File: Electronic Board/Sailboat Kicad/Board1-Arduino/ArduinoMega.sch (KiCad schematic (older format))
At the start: 7 parts, among them J2 Conn_01x08, J3 Conn_01x08, J4 Conn_01x08, J5 Conn_02x18_Odd_Even, J6 Conn_01x08, J7 Conn_01x08, J8 Conn_01x08

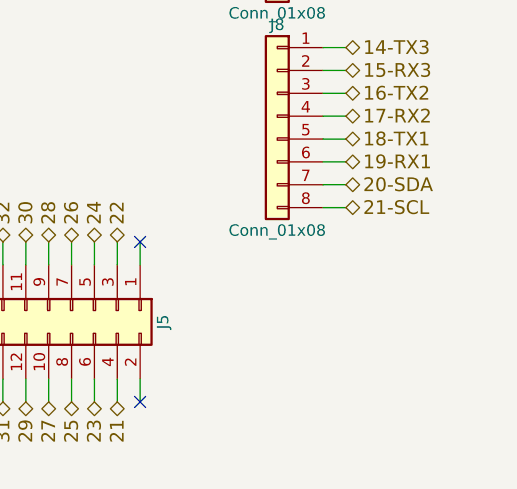
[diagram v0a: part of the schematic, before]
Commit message: Finished board-v0.1
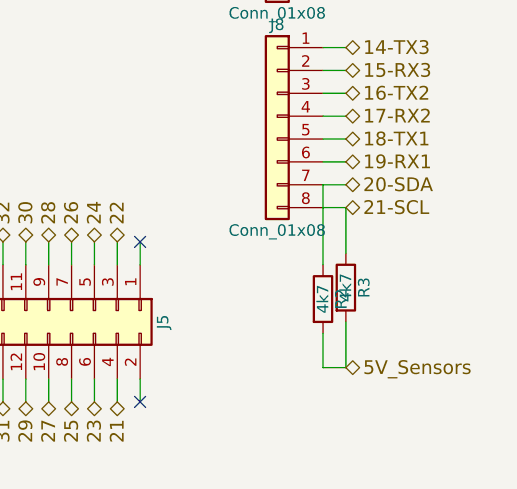
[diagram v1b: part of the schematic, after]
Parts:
- added R2, R3: 4k7, Resistors_THT:R_Axial_DIN0204_L3.6mm_D1.6mm_P7.62mm_Horizontal, symbol R
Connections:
- net 20-SDA: now also R2.1
- net 21-SCL: now also R3.1
- new net 5V_Sensors: R2.2, R3.2
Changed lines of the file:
@@
 NoConn ~ 6200 2900
 NoConn ~ 6200 2800
+$Comp
+L R R3
+U 1 1 5AB57136
+P 9500 5600
+F 0 "R3" V 9580 5600 50  0000 C CNN
+F 1 "4k7" V 9500 5600 50  0000 C CNN
+F 2 "Resistors_THT:R_Axial_DIN0204_L3.6mm_D1.6mm_P7.62mm_Horizontal" V 9430 5600 50  0001 C CNN
+F 3 "" H 9500 5600 50  0001 C CNN
+	1    9500 5600
+	1    0    0    -1
+$EndComp
+$Comp
+L R R2
+U 1 1 5AB57198
+P 9400 5650
+F 0 "R2" V 9480 5650 50  0000 C CNN
+F 1 "4k7" V 9400 5650 50  0000 C CNN
+F 2 "Resistors_THT:R_Axial_DIN0204_L3.6mm_D1.6mm_P7.62mm_Horizontal" V 9330 5650 50  0001 C CNN
+F 3 "" H 9400 5650 50  0001 C CNN
+	1    9400 5650
+	1    0    0    -1
+$EndComp
+Text HLabel 9500 5950 2    60   BiDi ~ 0
+5V_Sensors
+Wire Wire Line
+	9500 5750 9500 5950
+Wire Wire Line
+	9400 5800 9400 5950
+Wire Wire Line
+	9400 5950 9500 5950
+Wire Wire Line
+	9500 5450 9500 5250
+Wire Wire Line
+	9400 5500 9400 5150
 $EndSCHEMATC
